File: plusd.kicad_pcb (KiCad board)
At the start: 2 copper layers, 99.1 x 99.1 mm, 69 parts, among them IC1 WD1772, IC10 74LS27, IC11 GAL22V10, IC12 L7805, IC2 AT28C256, IC3 6264, IC4 GAL20V8, IC5 74LS06, IC6 74LS126, IC7 74LS374, IC8 74LS175, IC9 74LS00, J1 ZX_Spectrum_Connector_GENERIC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, J2 Conn_02x17_Odd_Even, J3 Conn_02x13_Odd_Even, J4 DB9_Male, SW1 SW_DPST_x2, SW2 SW_DPST_x2, SW3 SW_DIP_x03, Y1 8.000Mhz

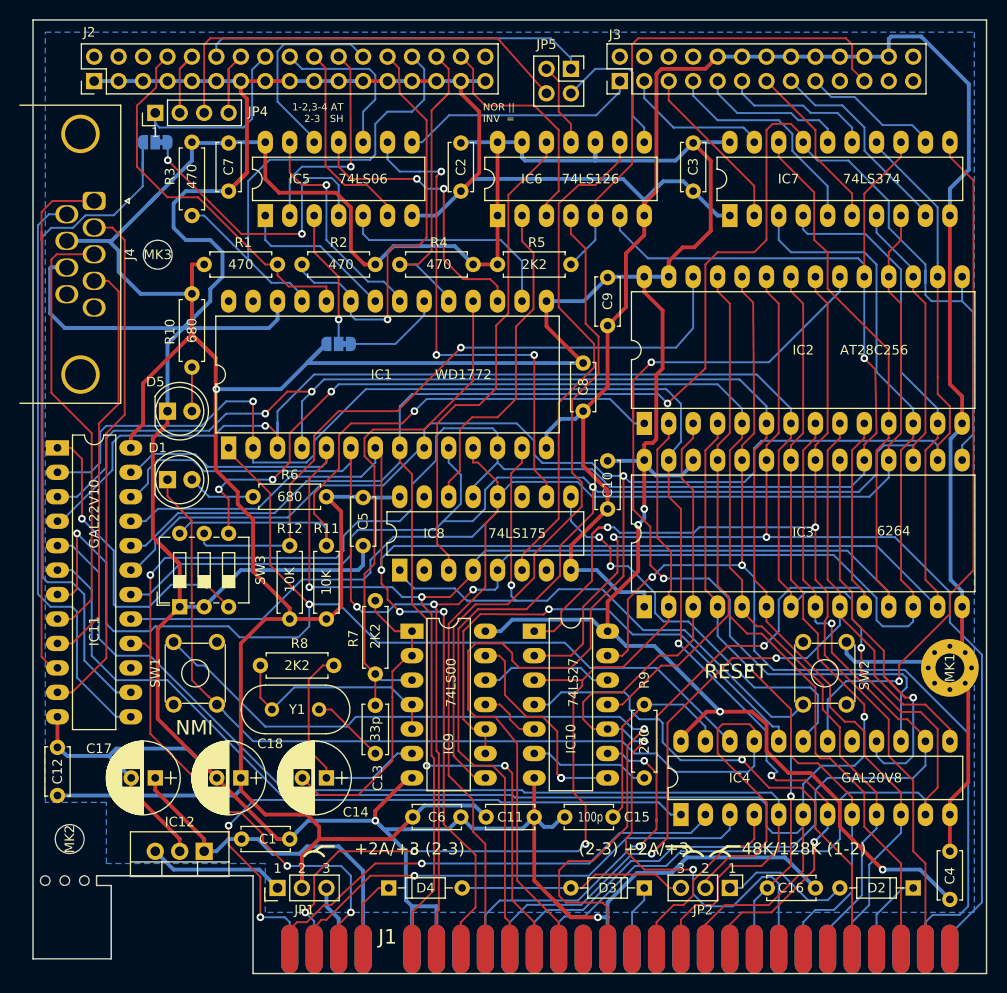
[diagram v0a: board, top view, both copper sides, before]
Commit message: añadido ibom
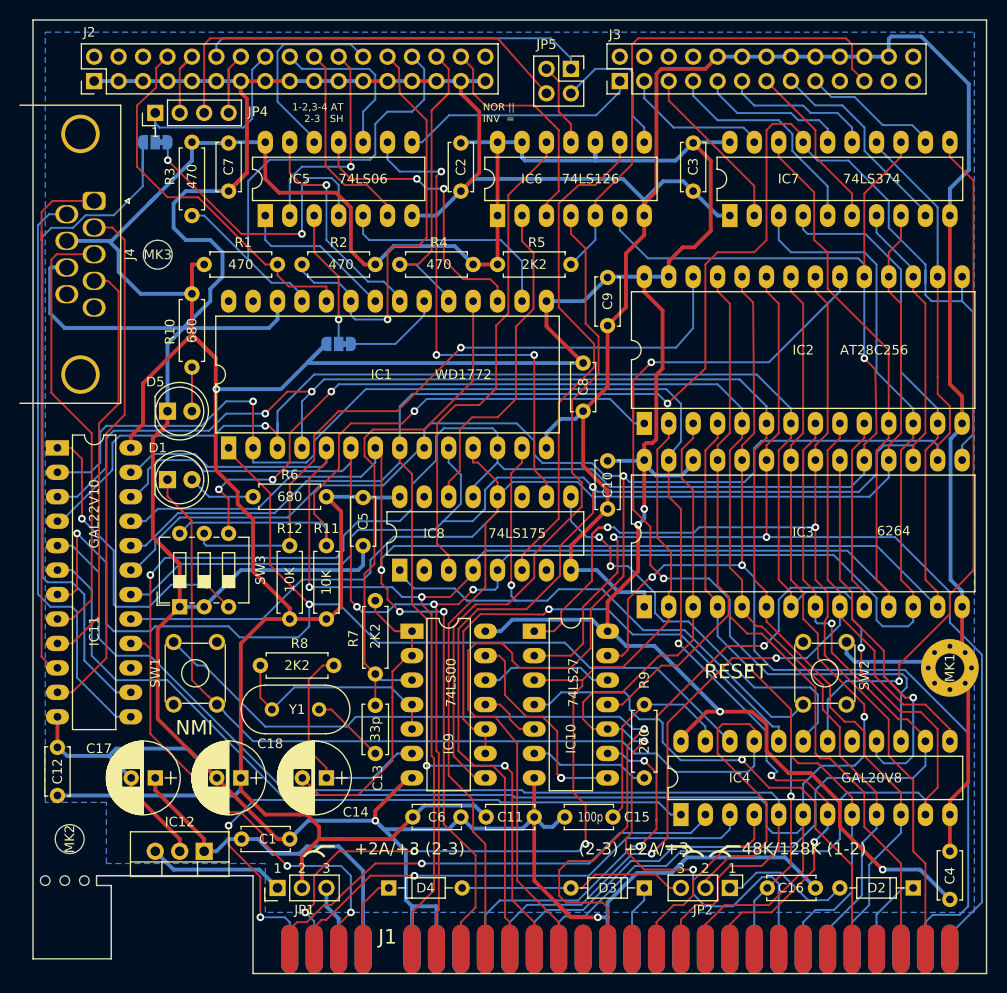
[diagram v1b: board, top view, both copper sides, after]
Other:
- net class Default removed
- net class power removed
